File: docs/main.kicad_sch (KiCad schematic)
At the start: 7 parts, among them Q1 IRLB8743

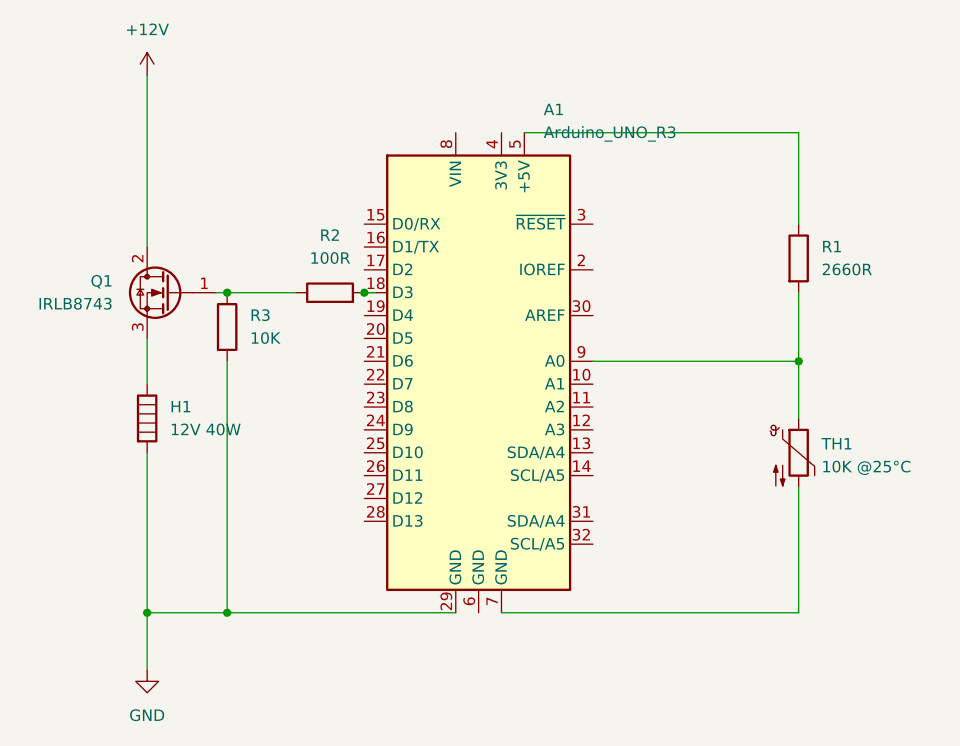
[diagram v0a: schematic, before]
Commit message: updated hardware
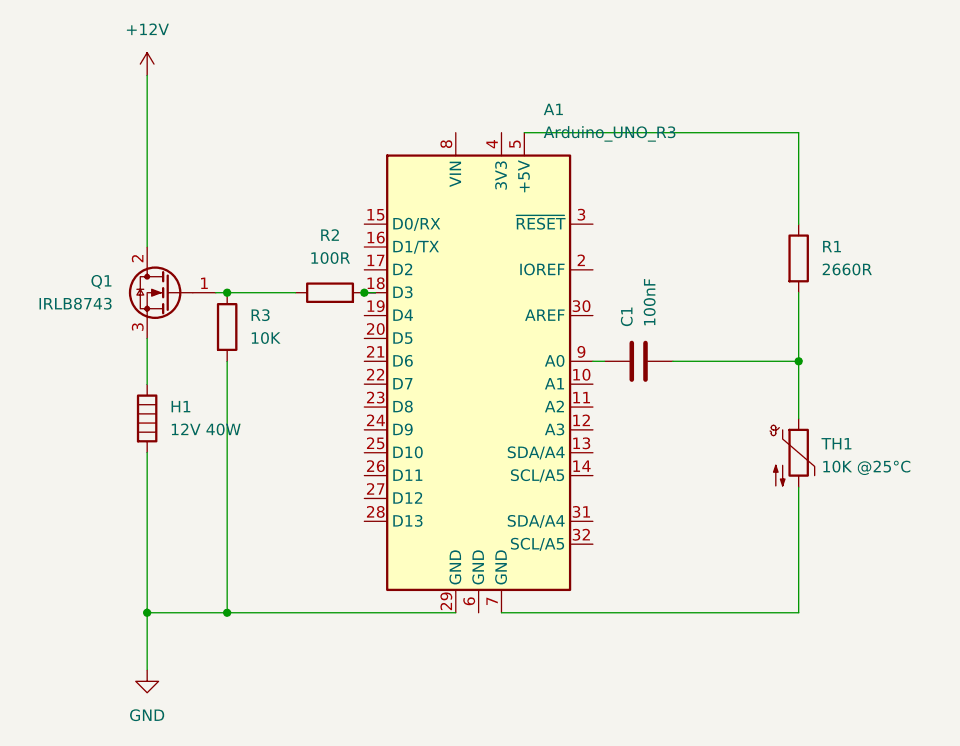
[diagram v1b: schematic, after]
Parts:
- added C1: 100nF, symbol Device:C
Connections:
- net at R1.2, TH1.1: now also C1.2; no longer A1.9 (A0)
- new net: A1.9 (A0), C1.1
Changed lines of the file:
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@@
 		(title "pid-temperature-controller|main")
 		(date "2026-05-13")
-		(rev "v1.1")
+		(rev "v1.2")
 	)
 	(junction
@@
 	(wire
 		(pts
-			(xy 133.35 81.28) (xy 156.21 81.28)
-		)
-		(stroke
-			(width 0)
-			(type default)
-		)
-	)
-	(wire
-		(pts
 			(xy 83.82 49.53) (xy 83.82 68.58)
 		)
@@
 	(wire
 		(pts
+			(xy 133.35 81.28) (xy 134.62 81.28)
+		)
+		(stroke
+			(width 0)
+			(type default)
+		)
+	)
+	(wire
+		(pts
 			(xy 92.71 81.28) (xy 92.71 109.22)
 		)
@@
 	(wire
 		(pts
+			(xy 142.24 81.28) (xy 156.21 81.28)
+		)
+		(stroke
+			(width 0)
+			(type default)
+		)
+	)
+	(wire
+		(pts
 			(xy 156.21 73.66) (xy 156.21 81.28)
 		)
@@
 	(wire
 		(pts
+			(xy 83.82 109.22) (xy 92.71 109.22)
+		)
+		(stroke
+			(width 0)
+			(type default)
+		)
+	)
+	(wire
+		(pts
+			(xy 83.82 91.44) (xy 83.82 109.22)
+		)
+		(stroke
+			(width 0)
+			(type default)
+		)
+	)
+	(wire
+		(pts
+			(xy 83.82 109.22) (xy 83.82 115.57)
+		)
+		(stroke
+			(width 0)
+			(type default)
+		)
+	)
+	(wire
+		(pts
+			(xy 92.71 73.66) (xy 100.33 73.66)
+		)
+		(stroke
+			(width 0)
+			(type default)
+		)
+	)
+	(wire
+		(pts
+			(xy 83.82 78.74) (xy 83.82 83.82)
+		)
+		(stroke
+			(width 0)
+			(type default)
+		)
+	)
+	(wire
+		(pts
+			(xy 125.73 55.88) (xy 156.21 55.88)
+		)
+		(stroke
+			(width 0)
+			(type default)
+		)
+	)
+	(wire
+		(pts
 			(xy 156.21 81.28) (xy 156.21 87.63)
-		)
-		(stroke
-			(width 0)
-			(type default)
-		)
-	)
-	(wire
-		(pts
-			(xy 83.82 109.22) (xy 92.71 109.22)
-		)
-		(stroke
-			(width 0)
-			(type default)
-		)
-	)
-	(wire
-		(pts
-			(xy 83.82 91.44) (xy 83.82 109.22)
-		)
-		(stroke
-			(width 0)
-			(type default)
-		)
-	)
-	(wire
-		(pts
-			(xy 83.82 109.22) (xy 83.82 115.57)
-		)
-		(stroke
-			(width 0)
-			(type default)
-		)
-	)
-	(wire
-		(pts
-			(xy 92.71 73.66) (xy 100.33 73.66)
-		)
-		(stroke
-			(width 0)
-			(type default)
-		)
-	)
-	(wire
-		(pts
-			(xy 83.82 78.74) (xy 83.82 83.82)
-		)
-		(stroke
-			(width 0)
-			(type default)
-		)
-	)
-	(wire
-		(pts
-			(xy 125.73 55.88) (xy 156.21 55.88)
 		)
 		(stroke
@@
 					(unit 1)
 				)
+			)
+		)
+	)
+	(symbol
+		(lib_id "Device:C")
+		(at 138.43 81.28 90)
+		(unit 1)
+		(body_style 1)
+		(exclude_from_sim no)
+		(in_bom yes)
+		(on_board yes)
+		(in_pos_files yes)
+		(dnp no)
+		(fields_autoplaced yes)
+		(property "Reference" "C1"
+			(at 137.1599 77.47 0)
+			(show_name no)
+			(do_not_autoplace no)
+			(effects
+				(font
+					(size 1.27 1.27)
+				)
+				(justify left)
+			)
+		)
+		(property "Value" "100nF"
+			(at 139.6999 77.47 0)
+			(show_name no)
+			(do_not_autoplace no)
+			(effects
+				(font
+					(size 1.27 1.27)
+				)
+				(justify left)
+			)
+		)
+		(property "Footprint" ""
+			(at 142.24 80.3148 0)
+			(hide yes)
+			(show_name no)
+			(do_not_autoplace no)
+			(effects
+				(font
+					(size 1.27 1.27)
+				)
+			)
+		)
+		(property "Datasheet" ""
+			(at 138.43 81.28 0)
+			(hide yes)
+			(show_name no)
+			(do_not_autoplace no)
+			(effects
+				(font
+					(size 1.27 1.27)
+				)
+			)
+		)
+		(property "Description" "Unpolarized capacitor"
+			(at 138.43 81.28 0)
+			(hide yes)
+			(show_name no)
+			(do_not_autoplace no)
+			(effects
+				(font
+					(size 1.27 1.27)
+				)
+			)
+		)
+		(pin "2"
+		)
+		(pin "1"
+		)
+		(instances
+			(project "main"
+				(path "/65a569c9-b81d-4fcf-906a-443098e8f4b2"
+					(reference "C1")
+					(unit 1)
+				)
